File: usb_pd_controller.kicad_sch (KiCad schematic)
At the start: 28 parts, among them Q1 BSS138, Q2 BSS138, Q3 IRF7855TRPBF, Q4 IRF7855TRPBF, U1 AP33772SDKZ-13-FA02

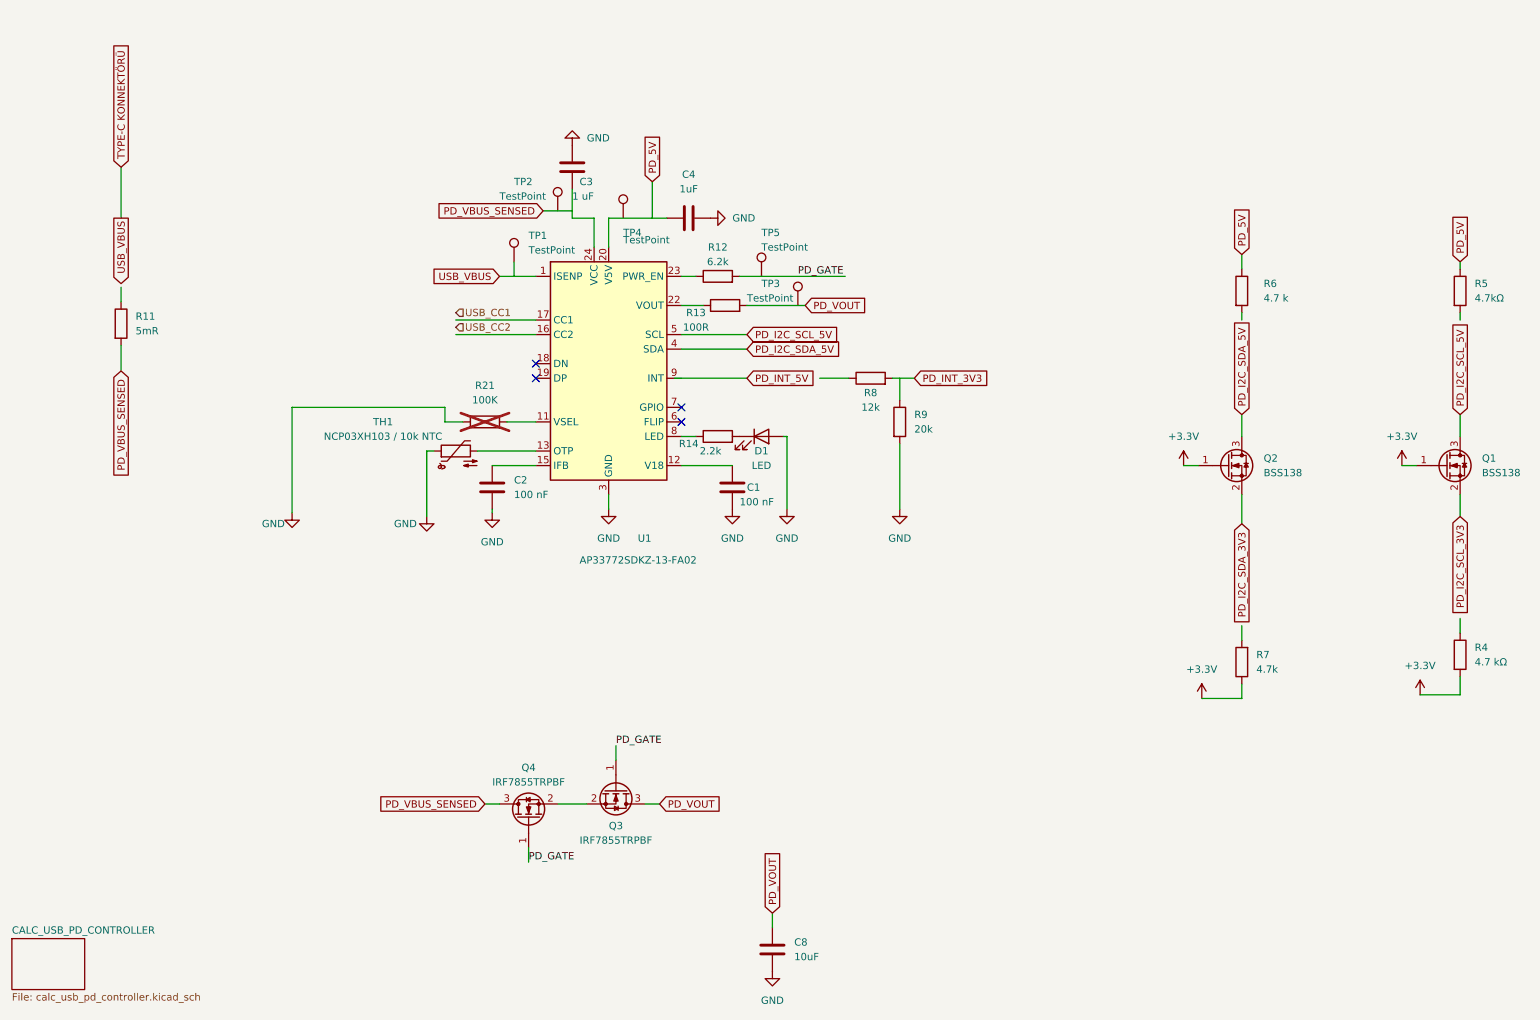
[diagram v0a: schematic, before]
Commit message: 10/09/26
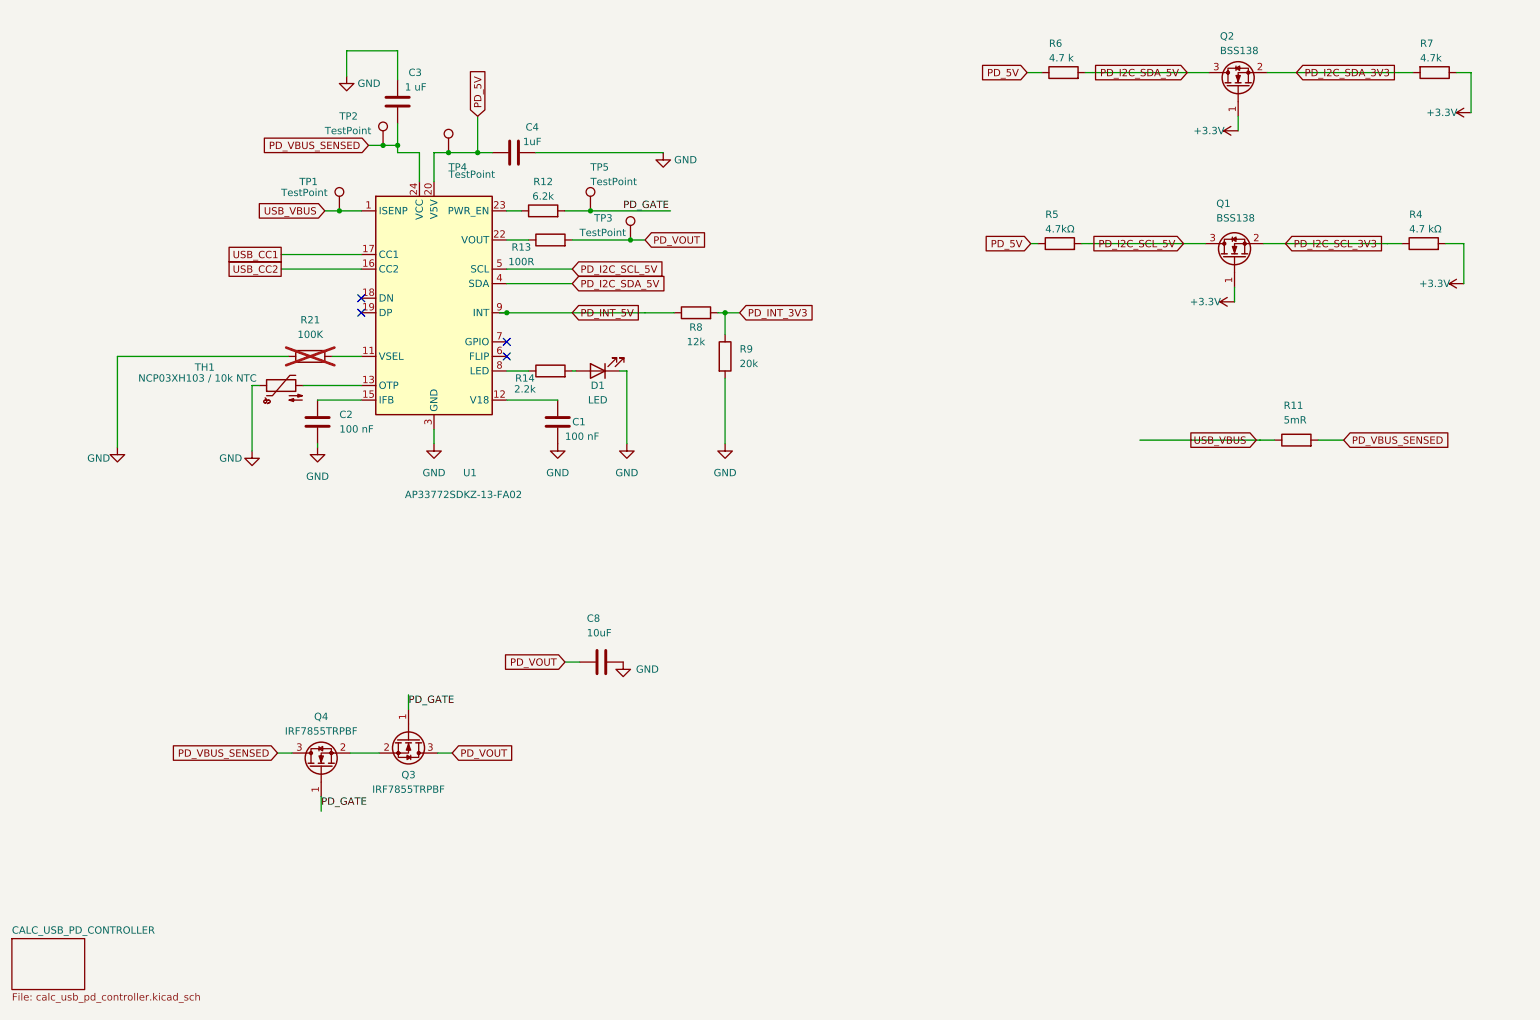
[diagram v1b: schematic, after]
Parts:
- R14, R8, R9: footprint Capacitor_SMD:C_01005_0402Metric -> Resistor_SMD:R_0603_1608Metric
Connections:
- net TYPE-C KONNEKTÖRÜ is gone; now on net USB_VBUS: U1.1 (ISENP)
- net GND: now also D1.1 (K); no longer D1.2 (A)
- net PD_5V: now also C4.1, TP4.1, U1.20 (V5V)
- net PD_GATE: now also TP5.1
- net PD_I2C_SCL_3V3: now also R4.1
- net PD_I2C_SCL_5V: now also R5.2
- net PD_I2C_SDA_3V3: now also R7.2
- net PD_I2C_SDA_5V: now also R6.2
- net PD_INT_3V3: now also R9.1
- net PD_INT_5V: now also R8.1, U1.9 (INT)
- net PD_VBUS_SENSED: now also C3.1, TP2.1, U1.24 (VCC)
- net PD_VOUT: now also TP3.1
- net USB_CC1: now also U1.17 (CC1)
- net USB_CC2: now also U1.16 (CC2)
- net USB_VBUS: now reaches TP1.1
- net USB_VBUS: now also R11.1
- net at R14.2: now also D1.2 (A); no longer D1.1 (K)
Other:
- moved on the sheet: C1, C2, C3, C4, C8, D1, Q1, Q2, Q3, Q4, R11, R12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
